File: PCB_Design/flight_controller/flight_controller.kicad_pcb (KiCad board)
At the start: 2 copper layers, 17 parts, among them J1 Screw_Terminal_01x02, J15 Conn_01x04, J16 Conn_01x04, J3 Conn_01x04, J4 Conn_01x03, J5 Conn_01x03, J6 Conn_01x03, J7 Conn_01x03, J8 Conn_01x05, U1 NUCLEO-F401RE

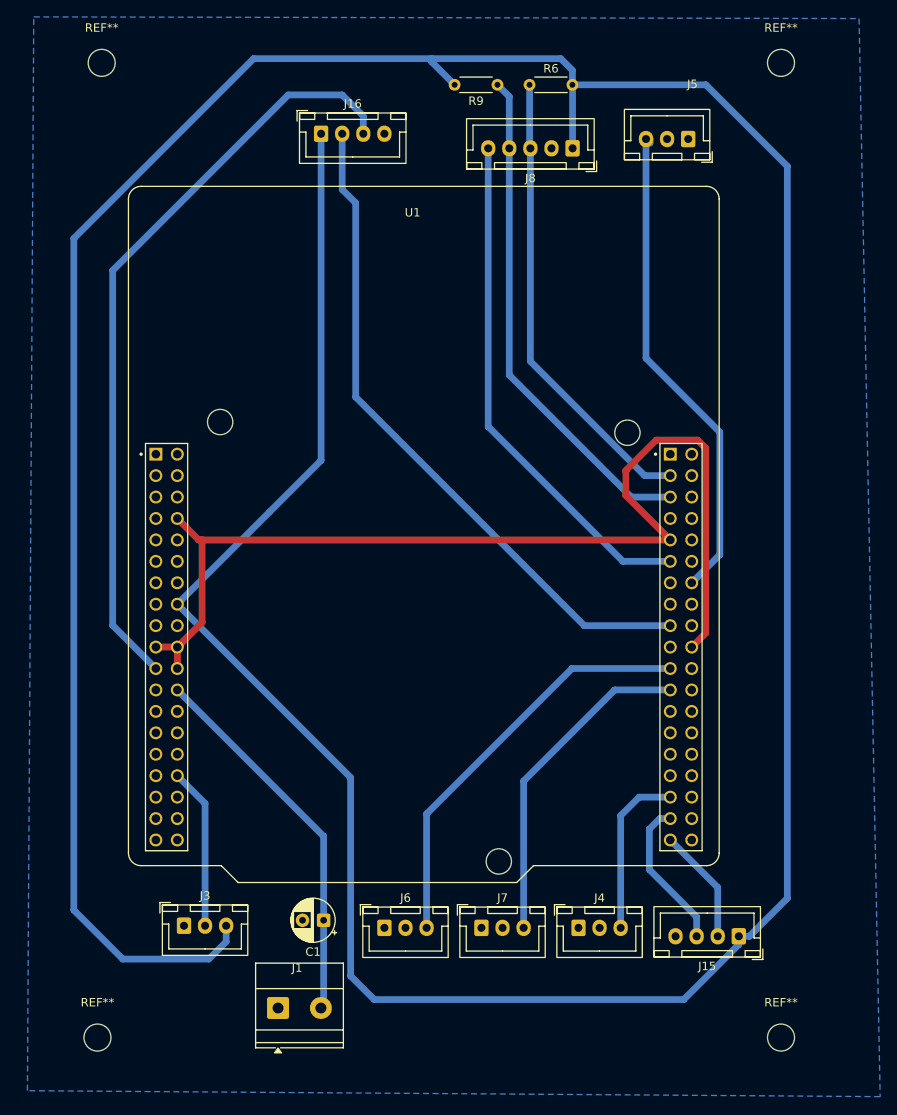
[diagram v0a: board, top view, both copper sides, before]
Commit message: new pcb
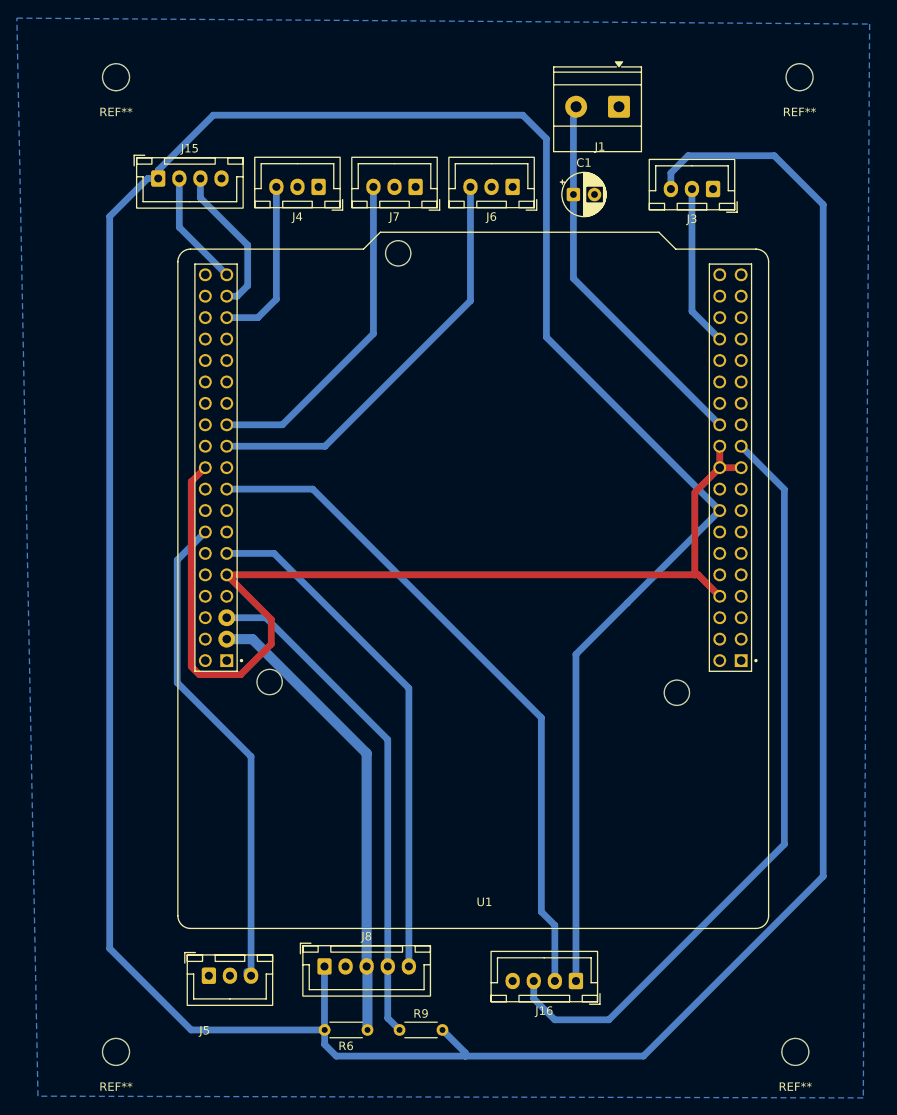
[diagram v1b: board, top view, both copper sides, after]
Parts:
- moved REF** 143.2 mm to (187.7, 142.2), turned to 180 degrees
- moved REF** 141.2 mm to (107.2, 142.2), turned to 180 degrees
- moved REF** 141.0 mm to (188.2, 26.7), turned to 180 degrees
- moved REF** 138.4 mm to (107.2, 26.7), turned to 180 degrees
- moved J5 114.3 mm to (118.2, 133.2), turned to 0 degrees
- moved J1 114.2 mm to (166.8, 30.2), turned to 180 degrees
- moved R6 113.6 mm to (137.0, 139.6), turned to 180 degrees
- moved J15 113.1 mm to (112.2, 38.7), turned to 0 degrees
- moved R9 112.6 mm to (140.8, 139.6), turned to 0 degrees
- moved J3 107.5 mm to (177.9, 40.0), turned to 180 degrees
- moved J16 104.8 mm to (161.7, 133.8), turned to 180 degrees
- moved J8 101.3 mm to (131.9, 132.1), turned to 0 degrees
- moved J4 93.0 mm to (131.2, 39.7), turned to 180 degrees
- moved C1 91.0 mm to (161.4, 40.6), turned to 0 degrees
- moved J6 89.1 mm to (154.2, 39.7), turned to 180 degrees
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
